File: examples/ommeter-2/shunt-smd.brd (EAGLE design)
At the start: 18 parts

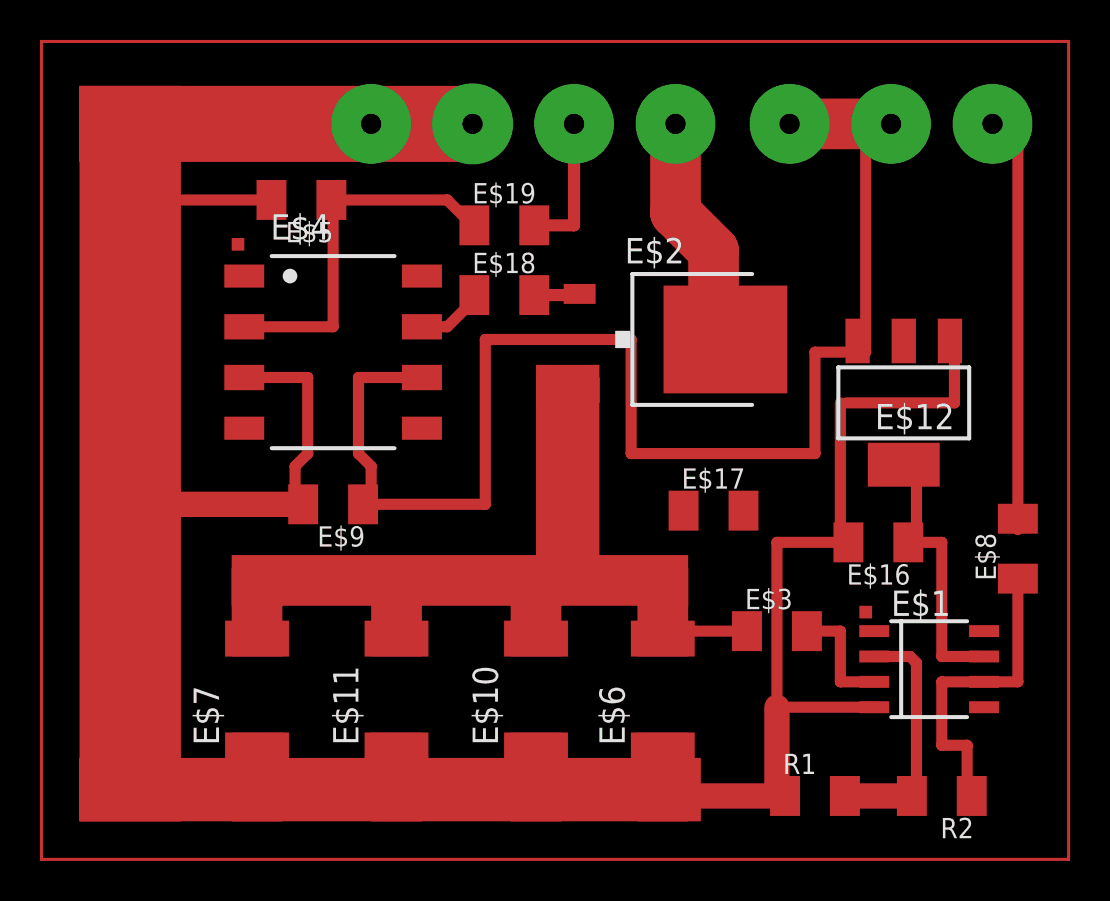
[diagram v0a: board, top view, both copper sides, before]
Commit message: Add files via upload
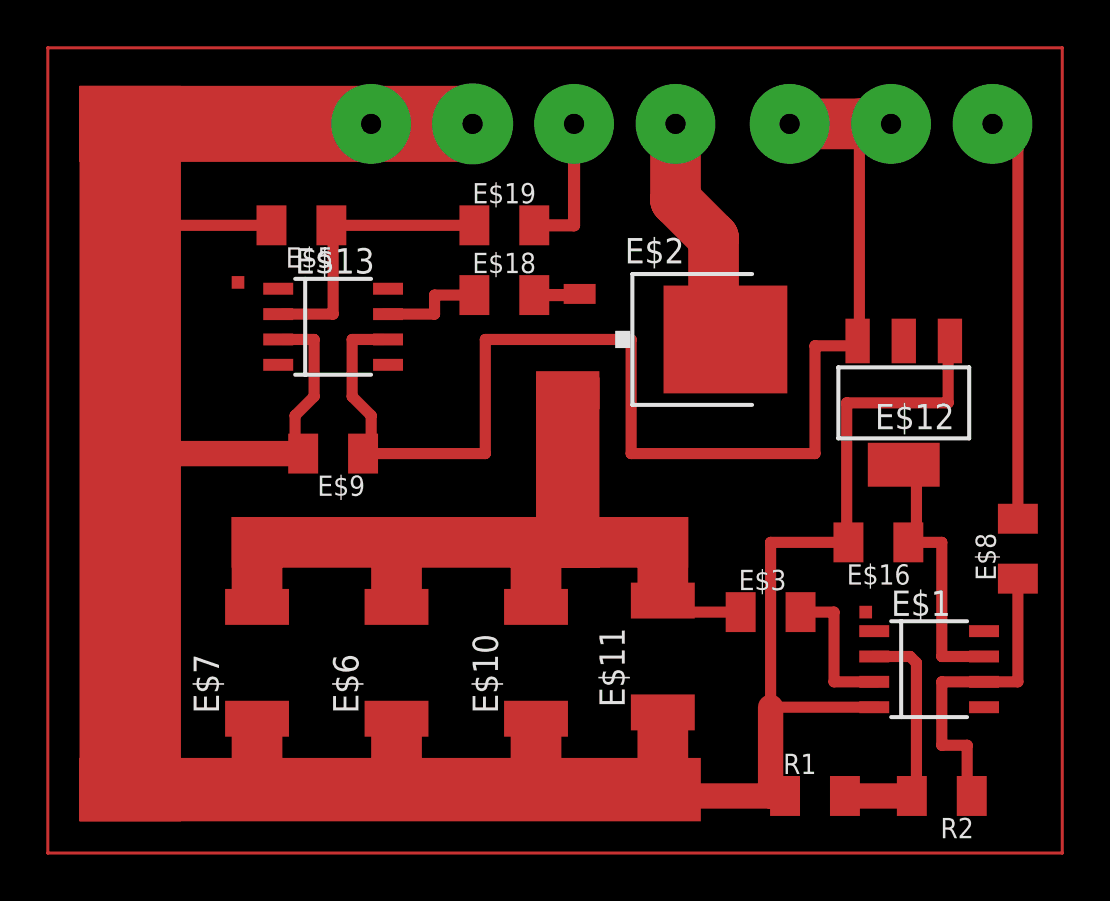
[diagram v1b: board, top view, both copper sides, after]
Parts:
- removed E$17: 1mk, rcl:C1206K
- removed E$4: IR4427, avago:DIP8
- added E$13: ir4427, linear:SOIC8
- moved E$11 13.5 mm to (31.8, 10.8)
- moved E$6 13.4 mm to (18.4, 10.5)
- moved E$9 2.54 mm to (15.2, 21.0)
- moved E$10 1.59 mm to (25.4, 10.5)
- moved E$7 1.59 mm to (11.4, 10.5)
- moved E$5 1.27 mm to (13.7, 32.4)
- moved E$3 1.00 mm to (37.1, 13.0)
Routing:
- net S$10: track 70.1 -> 65.2 mm
- net S$4: track 18.3 -> 14.0 mm
- net S$7: track 184.8 -> 182.2 mm
- net S$8: track 9.79 -> 7.70 mm
- net S$12: track 3.70 -> 5.40 mm
- net S$9: track 5.72 -> 6.98 mm
- net S$6: track 32.4 -> 33.0 mm
- net S$16: track 20.8 -> 20.2 mm
